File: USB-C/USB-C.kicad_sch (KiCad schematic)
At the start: 6 parts, among them J1 USB_C_Receptacle_USB2.0

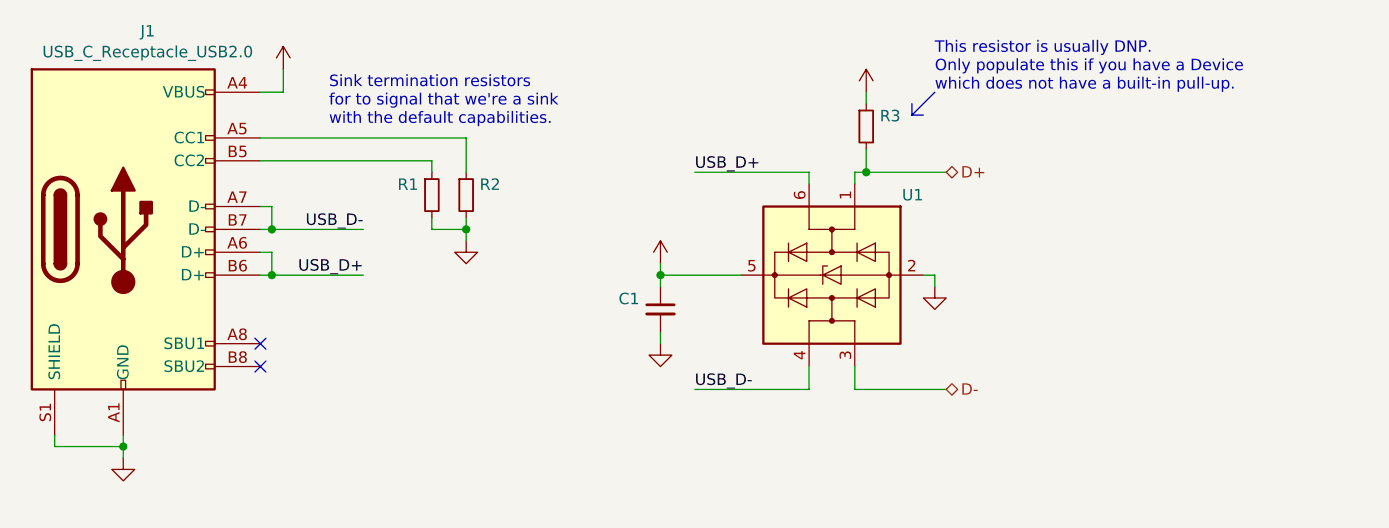
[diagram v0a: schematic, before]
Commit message: Reapply "Update modules to kicad v7 format"
This reverts commit fa5cc85431189ac7a3beedf0871b5723203ae43f.
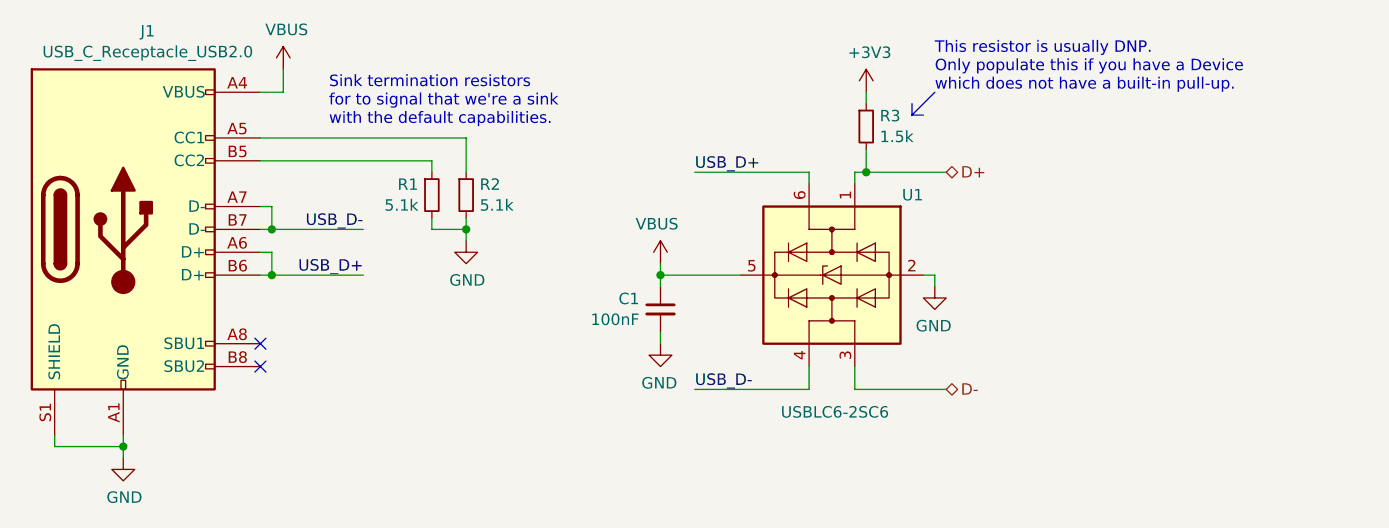
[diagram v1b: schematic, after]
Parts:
- C1: value (none) -> 100nF; footprint (none) -> Capacitor_SMD:C_0402_1005Metric
- R1, R2: value (none) -> 5.1k; footprint (none) -> Resistor_SMD:R_0402_1005Metric
- R3: value (none) -> 1.5k; footprint (none) -> Resistor_SMD:R_0603_1608Metric
- U1: value (none) -> USBLC6-2SC6; footprint (none) -> Package_TO_SOT_SMD:SOT-23-6
